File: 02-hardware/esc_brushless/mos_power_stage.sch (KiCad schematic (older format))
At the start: 18 parts

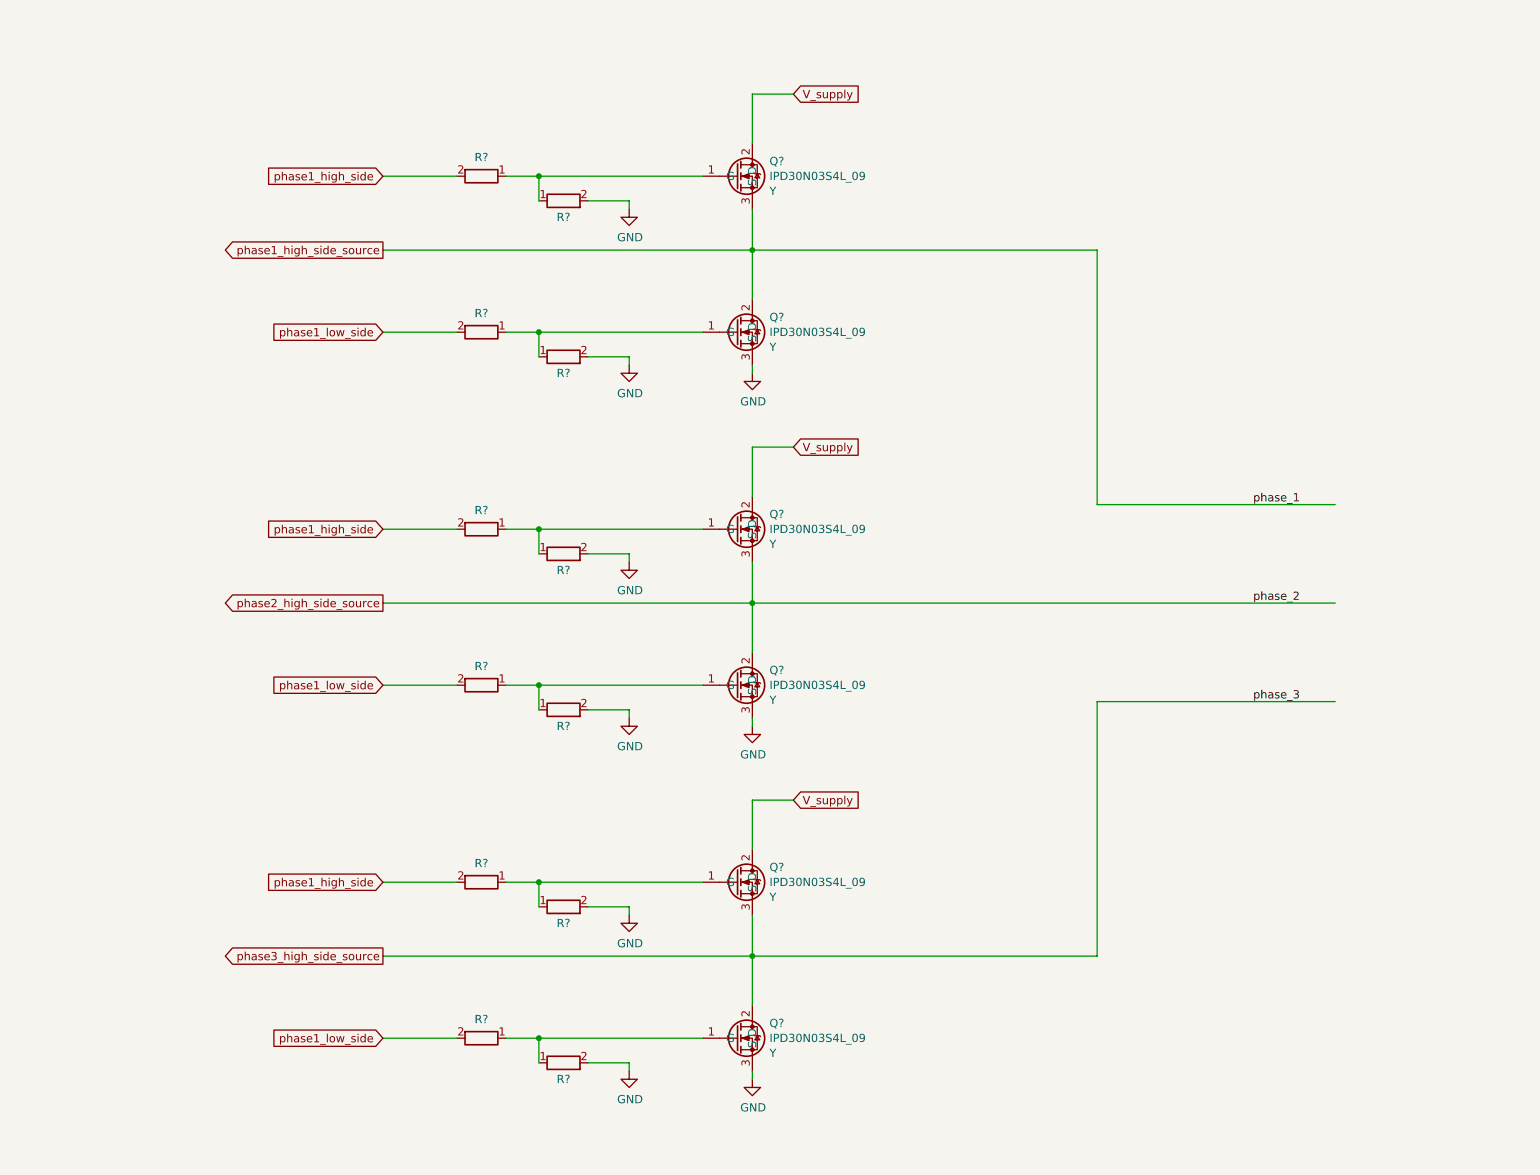
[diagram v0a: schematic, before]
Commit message: Schematics v1.0 - Architecture V1.0, fix DRC issues
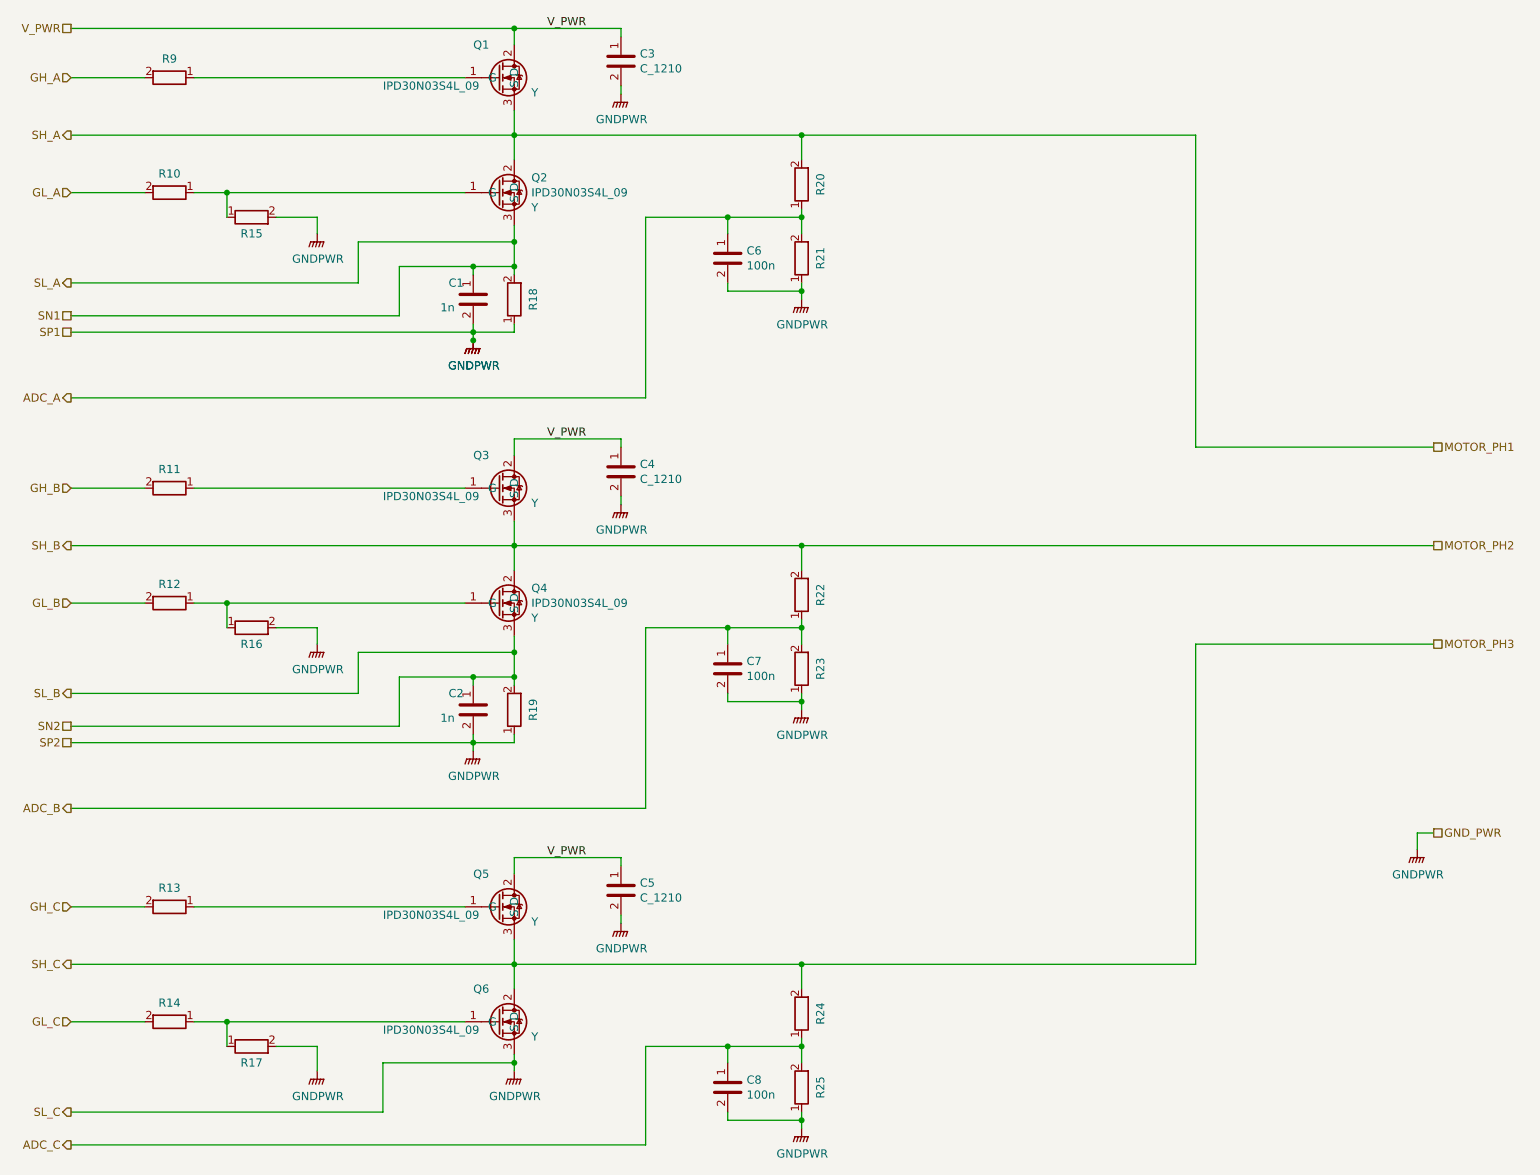
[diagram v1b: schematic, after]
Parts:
- removed Q? (x2): IPD30N03S4L_09, p_Package_TO_SMD:TO-252-pin_1_3_TabPin2, symbol p_Transistor_FET:IPD30N03S4L_09
- removed R? (x3): R_0603, p_Package_Resistor_SMD:R_0603_1608Metric_Pad0.98x0.95mm_HandSolder, symbol p_Passive:R_0603
- added C1, C2: 1n, p_Package_Capacitor_SMD:C_0603_1608Metric_Pad1.08x0.95mm_HandSolder, symbol p_Passive:C_0603
- added C3, C4, C5: C_1210, p_Package_Capacitor_SMD:C_1210_3225Metric_Pad1.33x2.70mm_HandSolder, symbol p_Passive:C_1210
- added C6, C7, C8: 100n, p_Package_Capacitor_SMD:C_0805_2012Metric_Pad1.18x1.45mm_HandSolder, symbol p_Passive:C_0805
- added Q1, Q3: IPD30N03S4L_09, p_Package_TO_SMD:TO-252-pin_1_3_TabPin2, symbol p_Transistor_FET:IPD30N03S4L_09
- added R18, R19, R20, R21, R22, R23, R24, R25: R_0603, p_Package_Resistor_SMD:R_0603_1608Metric_Pad0.98x0.95mm_HandSolder, symbol p_Passive:R_0603
- gave numbers to parts that had none: 13
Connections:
- net labels added: ADC_A, ADC_B, ADC_C, GH_A, GH_B, GH_C, GL_A, GL_B, GL_C, GNDPWR, GND_PWR, MOTOR_PH1, MOTOR_PH2, MOTOR_PH3, SH_A, SH_B, SH_C, SL_A, SL_B, SL_C, SN1, SN2, SP1, SP2, V_PWR
- net labels removed: GND, V_supply, phase1_high_side, phase1_high_side_source, phase1_low_side, phase2_high_side_source, phase3_high_side_source, phase_1, phase_2, phase_3
- wire segments 61 -> 131
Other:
- moved on the sheet: Q2, Q4, Q5, Q6, R10, R11, R12, R13, R14, R15, R16, R17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
